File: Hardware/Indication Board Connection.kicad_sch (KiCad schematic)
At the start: 16 parts, among them J18 Conn_01x03, U11 TPS5405DR

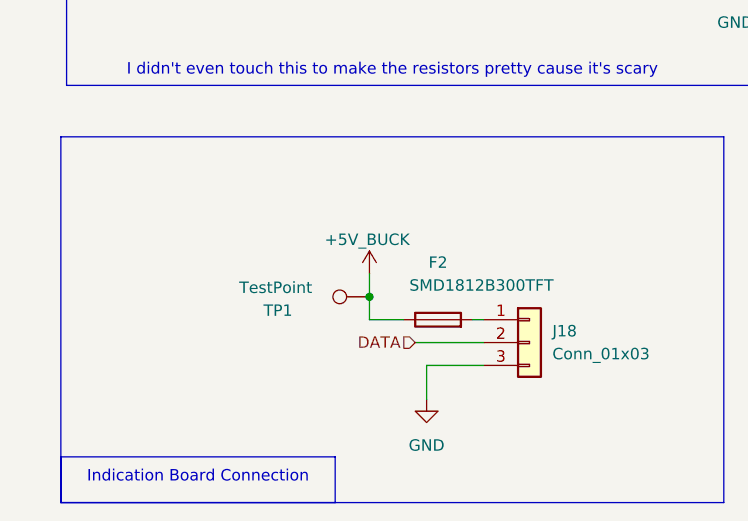
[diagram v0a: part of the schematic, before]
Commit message: Backup
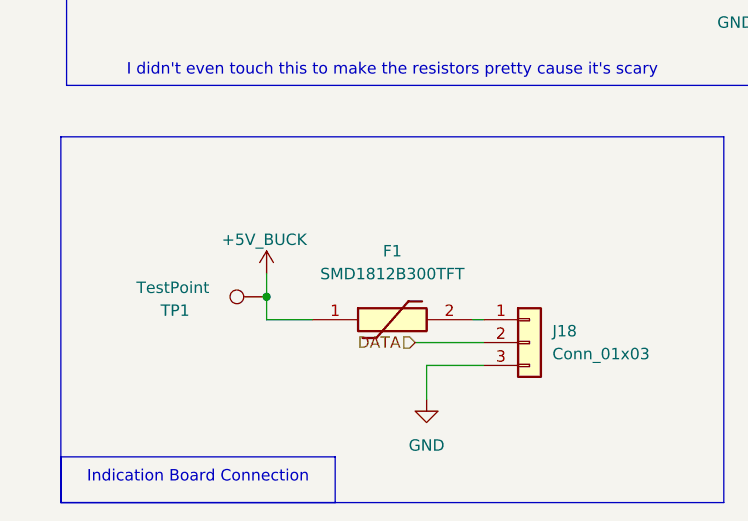
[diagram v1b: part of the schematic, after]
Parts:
- removed F2: SMD1812B300TFT, Fuse:Fuse_1812_4532Metric, symbol Device:Fuse
- added F1: SMD1812B300TFT, PTC Fuse:FUSC4632X165N, symbol PTC Fuse:SMD1812B300TFT
- J18: footprint Connector_Molex:Molex_Nano-Fit_105309-xx03_1x03_P2.50mm_Vertical -> Connector_Molex:Molex_Nano-Fit_105313-xx03_1x03_P2.50mm_Horizontal
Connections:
- net +5V_BUCK: now also F1.1
- net at J18.1 (Pin_1): now also F1.2
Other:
- moved on the sheet: TP1
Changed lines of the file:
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@@
 	)
 	(junction
-		(at 59.69 137.16)
+		(at 48.26 137.16)
 		(diameter 0)
 		(color 0 0 0 0)
@@
 	(wire
 		(pts
-			(xy 59.69 139.7) (xy 63.5 139.7)
+			(xy 48.26 139.7) (xy 53.34 139.7)
 		)
 		(stroke
@@
 	(wire
 		(pts
-			(xy 59.69 134.62) (xy 59.69 137.16)
+			(xy 48.26 134.62) (xy 48.26 137.16)
 		)
 		(stroke
@@
 	(wire
 		(pts
-			(xy 59.69 137.16) (xy 59.69 139.7)
+			(xy 48.26 137.16) (xy 48.26 139.7)
 		)
 		(stroke
@@
 	)
 	(symbol
-		(lib_id "Device:Fuse")
-		(at 67.31 139.7 90)
+		(lib_id "power:GND")
+		(at 142.24 83.82 0)
 		(unit 1)
 		(exclude_from_sim no)
@@
 		(on_board yes)
 		(dnp no)
-		(property "Reference" "F2"
-			(at 67.31 133.35 90)
-			(effects
-				(font
-					(size 1.27 1.27)
-				)
-			)
-		)
-		(property "Value" "SMD1812B300TFT"
-			(at 72.136 135.89 90)
+		(fields_autoplaced yes)
+		(property "Reference" "#PWR0129"
+			(at 142.24 90.17 0)
 			(effects
 				(font
 					(size 1.27 1.27)
 				)
+				(hide yes)
 			)
 		)
-		(property "Footprint" "Fuse:Fuse_1812_4532Metric"
-			(at 67.31 141.478 90)
+		(property "Value" "GND"
+			(at 142.24 88.9 0)
 			(effects
 				(font
 					(size 1.27 1.27)
 				)
-				(hide yes)
 			)
 		)
-		(property "Datasheet" "https://4donline.ihs.com/images/VipMasterIC/IC/YAGO/YAGO-S-A0012927858/YAGO-S-A0012927859-1.pdf?hkey=CECEF36DEECDED6468708AAF2E19C0C6"
-			(at 67.31 139.7 0)
+		(property "Footprint" ""
+			(at 142.24 83.82 0)
 			(effects
 				(font
@@
 			)
 		)
-		(property "Description" "PPTC Fuse"
-			(at 67.31 139.7 0)
+		(property "Datasheet" ""
+			(at 142.24 83.82 0)
 			(effects
 				(font
@@
 			)
 		)
-		(property "Manufactuerer" ""
-			(at 67.31 139.7 90)
+		(property "Description" "Power symbol creates a global label with name \"GND\" , ground"
+			(at 142.24 83.82 0)
 			(effects
 				(font
@@
 			)
 		)
-		(pin "2"
-		)
 		(pin "1"
 		)
 		(instances
-			(project ""
+			(project "BPS-Leader"
 				(path "/fb37da34-e420-4994-8cc1-079e8c0fa48e/e5707b84-df8b-4b8b-b215-90bb9859c3b3"
-					(reference "F2")
+					(reference "#PWR0129")
 					(unit 1)
 				)
@@
 	)
 	(symbol
-		(lib_id "power:GND")
-		(at 142.24 83.82 0)
+		(lib_id "power:+24V")
+		(at 63.5 58.42 0)
 		(unit 1)
 		(exclude_from_sim no)
@@
 		(dnp no)
 		(fields_autoplaced yes)
-		(property "Reference" "#PWR0129"
-			(at 142.24 90.17 0)
+		(property "Reference" "#PWR0124"
+			(at 63.5 62.23 0)
 			(effects
 				(font
@@
 			)
 		)
-		(property "Value" "GND"
-			(at 142.24 88.9 0)
+		(property "Value" "+24V"
+			(at 63.5 53.34 0)
 			(effects
 				(font
@@
 		)
 		(property "Footprint" ""
-			(at 142.24 83.82 0)
+			(at 63.5 58.42 0)
 			(effects
 				(font
@@
 		)
 		(property "Datasheet" ""
-			(at 142.24 83.82 0)
+			(at 63.5 58.42 0)
 			(effects
 				(font
@@
 			)
 		)
-		(property "Description" "Power symbol creates a global label with name \"GND\" , ground"
-			(at 142.24 83.82 0)
+		(property "Description" "Power symbol creates a global label with name \"+24V\""
+			(at 63.5 58.42 0)
 			(effects
 				(font
@@
 			(project "BPS-Leader"
 				(path "/fb37da34-e420-4994-8cc1-079e8c0fa48e/e5707b84-df8b-4b8b-b215-90bb9859c3b3"
-					(reference "#PWR0129")
+					(reference "#PWR0124")
 					(unit 1)
 				)
@@
 	)
 	(symbol
-		(lib_id "power:+24V")
-		(at 63.5 58.42 0)
+		(lib_id "power:GND")
+		(at 63.5 81.28 0)
 		(unit 1)
 		(exclude_from_sim no)
@@
 		(on_board yes)
 		(dnp no)
-		(fields_autoplaced yes)
-		(property "Reference" "#PWR0124"
-			(at 63.5 62.23 0)
+		(property "Reference" "#PWR0125"
+			(at 63.5 87.63 0)
 			(effects
 				(font
@@
 			)
 		)
-		(property "Value" "+24V"
-			(at 63.5 53.34 0)
+		(property "Value" "GND"
+			(at 63.5 86.36 0)
 			(effects
 				(font
@@
 		)
 		(property "Footprint" ""
-			(at 63.5 58.42 0)
+			(at 63.5 81.28 0)
 			(effects
 				(font
@@
 		)
 		(property "Datasheet" ""
-			(at 63.5 58.42 0)
+			(at 63.5 81.28 0)
 			(effects
 				(font
@@
 			)
 		)
-		(property "Description" "Power symbol creates a global label with name \"+24V\""
-			(at 63.5 58.42 0)
+		(property "Description" "Power symbol creates a global label with name \"GND\" , ground"
+			(at 63.5 81.28 0)
 			(effects
 				(font
@@
 			(project "BPS-Leader"
 				(path "/fb37da34-e420-4994-8cc1-079e8c0fa48e/e5707b84-df8b-4b8b-b215-90bb9859c3b3"
-					(reference "#PWR0124")
+					(reference "#PWR0125")
 					(unit 1)
 				)
@@
 	)
 	(symbol
-		(lib_id "power:GND")
-		(at 63.5 81.28 0)
+		(lib_id "PTC Fuse:SMD1812B300TFT")
+		(at 53.34 139.7 0)
 		(unit 1)
 		(exclude_from_sim no)
@@
 		(on_board yes)
 		(dnp no)
-		(property "Reference" "#PWR0125"
-			(at 63.5 87.63 0)
+		(fields_autoplaced yes)
+		(property "Reference" "F1"
+			(at 62.23 132.08 0)
+			(effects
+				(font
+					(size 1.27 1.27)
+				)
+			)
+		)
+		(property "Value" "SMD1812B300TFT"
+			(at 62.23 134.62 0)
+			(effects
+				(font
+					(size 1.27 1.27)
+				)
+			)
+		)
+		(property "Footprint" "PTC Fuse:FUSC4632X165N"
+			(at 67.31 235.89 0)
 			(effects
 				(font
 					(size 1.27 1.27)
 				)
+				(justify left top)
 				(hide yes)
 			)
 		)
-		(property "Value" "GND"
-			(at 63.5 86.36 0)
+		(property "Datasheet" "https://www.yageo.com/upload/media/product/productsearch/datasheet/cpc/pptc/SMD1812_1.pdf"
+			(at 67.31 335.89 0)
 			(effects
 				(font
 					(size 1.27 1.27)
 				)
+				(justify left top)
+				(hide yes)
 			)
 		)
-		(property "Footprint" ""
-			(at 63.5 81.28 0)
+		(property "Description" "Polymeric PTC Resettable Fuse 6V 3 A Ih Surface Mount 1812 (4532 Metric), Concave"
+			(at 53.34 139.7 0)
 			(effects
 				(font
@@
 			)
 		)
-		(property "Datasheet" ""
-			(at 63.5 81.28 0)
+		(property "Height" "1.65"
+			(at 67.31 535.89 0)
 			(effects
 				(font
 					(size 1.27 1.27)
 				)
+				(justify left top)
 				(hide yes)
 			)
 		)
-		(property "Description" "Power symbol creates a global label with name \"GND\" , ground"
-			(at 63.5 81.28 0)
+		(property "Mouser Part Number" "603-SMD1812B300TFT"
+			(at 67.31 635.89 0)
+			(effects
+				(font
+					(size 1.27 1.27)
+				)
+				(justify left top)
+				(hide yes)
+			)
+		)
+		(property "Mouser Price/Stock" "https://www.mouser.co.uk/ProductDetail/YAGEO/SMD1812B300TFT?qs=0lSvoLzn4L%252BUTwukZpvWFw%3D%3D"
+			(at 67.31 735.89 0)
 			(effects
 				(font
 					(size 1.27 1.27)
 				)
+				(justify left top)
 				(hide yes)
 			)
 		)
+		(property "Manufacturer_Name" "YAGEO"
+			(at 67.31 835.89 0)
+			(effects
+				(font
+					(size 1.27 1.27)
+				)
+				(justify left top)
+				(hide yes)
+			)
+		)
+		(property "Manufacturer_Part_Number" "SMD1812B300TFT"
+			(at 67.31 935.89 0)
+			(effects
+				(font
+					(size 1.27 1.27)
+				)
+				(justify left top)
+				(hide yes)
+			)
+		)
+		(pin "2"
+		)
 		(pin "1"
 		)
 		(instances
-			(project "BPS-Leader"
+			(project ""
 				(path "/fb37da34-e420-4994-8cc1-079e8c0fa48e/e5707b84-df8b-4b8b-b215-90bb9859c3b3"
-					(reference "#PWR0125")
+					(reference "F1")
 					(unit 1)
 				)
@@
 	(symbol
 		(lib_id "power:+24V")
-		(at 59.69 134.62 0)
+		(at 48.26 134.62 0)
 		(unit 1)
 		(exclude_from_sim no)
@@
 		(dnp no)
 		(property "Reference" "#PWR0131"
-			(at 59.69 138.43 0)
+			(at 48.26 138.43 0)
 			(effects
 				(font
@@
 		)
 		(property "Value" "+5V_BUCK"
-			(at 59.436 130.81 0)
+			(at 48.006 130.81 0)
 			(effects
 				(font
@@
 		)
 		(property "Footprint" ""
-			(at 59.69 134.62 0)
+			(at 48.26 134.62 0)
 			(effects
 				(font
@@
 		)
 		(property "Datasheet" ""
-			(at 59.69 134.62 0)
+			(at 48.26 134.62 0)
 			(effects
 				(font
@@
 		)
 		(property "Description" "Power symbol creates a global label with name \"+24V\""
-			(at 59.69 134.62 0)
+			(at 48.26 134.62 0)
 			(effects
 				(font
@@
 	(symbol
 		(lib_id "Connector:TestPoint")
-		(at 59.69 137.16 90)
+		(at 48.26 137.16 90)
 		(unit 1)
 		(exclude_from_sim no)
@@
 		(dnp no)
 		(property "Reference" "TP1"
-			(at 49.53 138.684 90)
+			(at 38.1 138.684 90)
 			(effects
 				(font
@@
 		)
 		(property "Value" "TestPoint"
-			(at 49.276 136.144 90)
+			(at 37.846 136.144 90)
 			(effects
 				(font
@@
 		)
 		(property "Footprint" "TestPoint:TestPoint_Pad_1.0x1.0mm"
-			(at 59.69 132.08 0)
+			(at 48.26 132.08 0)
 			(effects
 				(font
@@
 		)
 		(property "Datasheet" "~"
-			(at 59.69 132.08 0)
+			(at 48.26 132.08 0)
 			(effects
 				(font
@@
 		)
 		(property "Description" "test point"
-			(at 59.69 137.16 0)
+			(at 48.26 137.16 0)
 			(effects
 				(font
@@
 		)
 		(property "Manufactuerer" ""
-			(at 59.69 137.16 90)
+			(at 48.26 137.16 90)
 			(effects
 				(font
@@
 			)
 		)
-		(property "Footprint" "Connector_Molex:Molex_Nano-Fit_105309-xx03_1x03_P2.50mm_Vertical"
+		(property "Footprint" "Connector_Molex:Molex_Nano-Fit_105313-xx03_1x03_P2.50mm_Horizontal"
 			(at 77.47 142.24 0)
 			(effects
